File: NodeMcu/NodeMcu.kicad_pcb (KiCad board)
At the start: 2 copper layers, 8.2 x 5 mm, 38 parts, among them J1 Conn_01x15_Male, J2 Conn_01x15_Male, P1 USB_C_Plug_USB2.0, Q1 Q_Dual_NPN_NPN_E1B1C2E2B2C1, SW1 SW_Push, SW2 SW_Push, U1 ESP-12E, U2 SPX3819M5-L-3-3, U3 CH340C

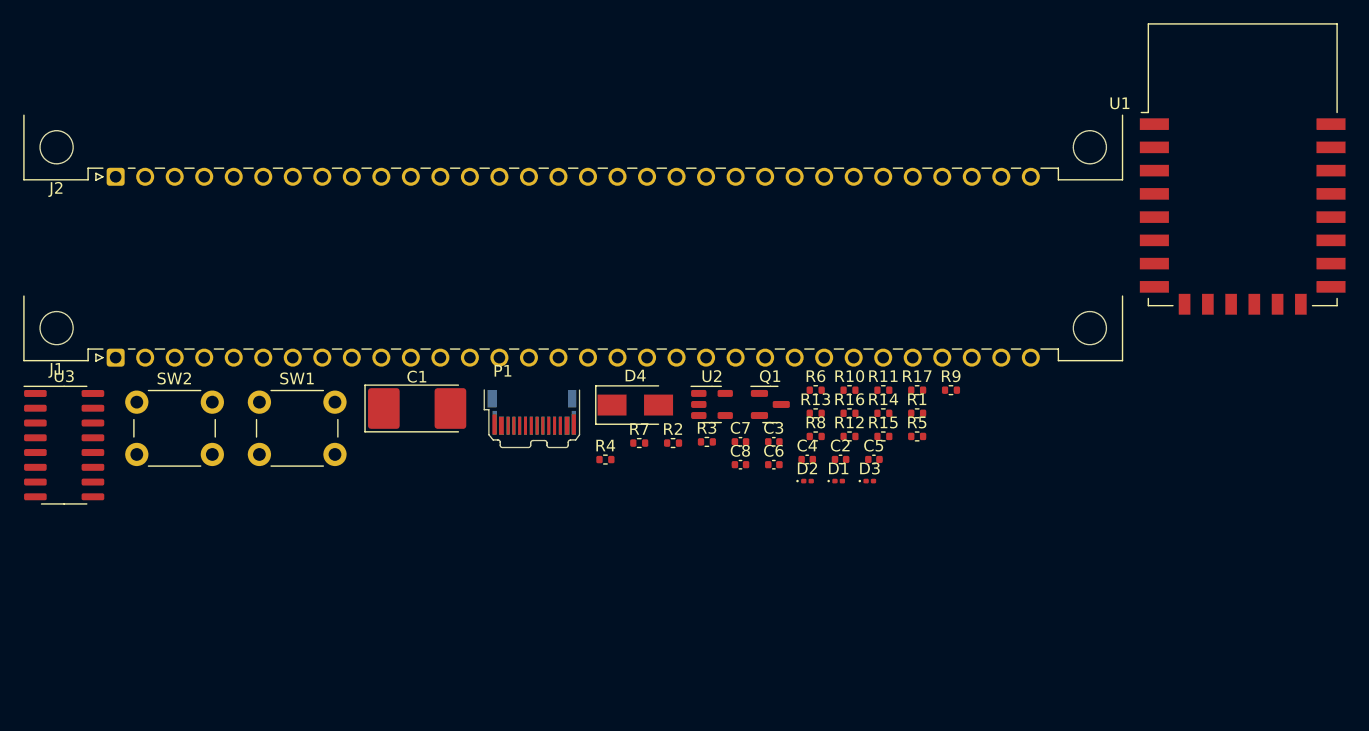
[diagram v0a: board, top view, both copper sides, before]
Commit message: nodemcu
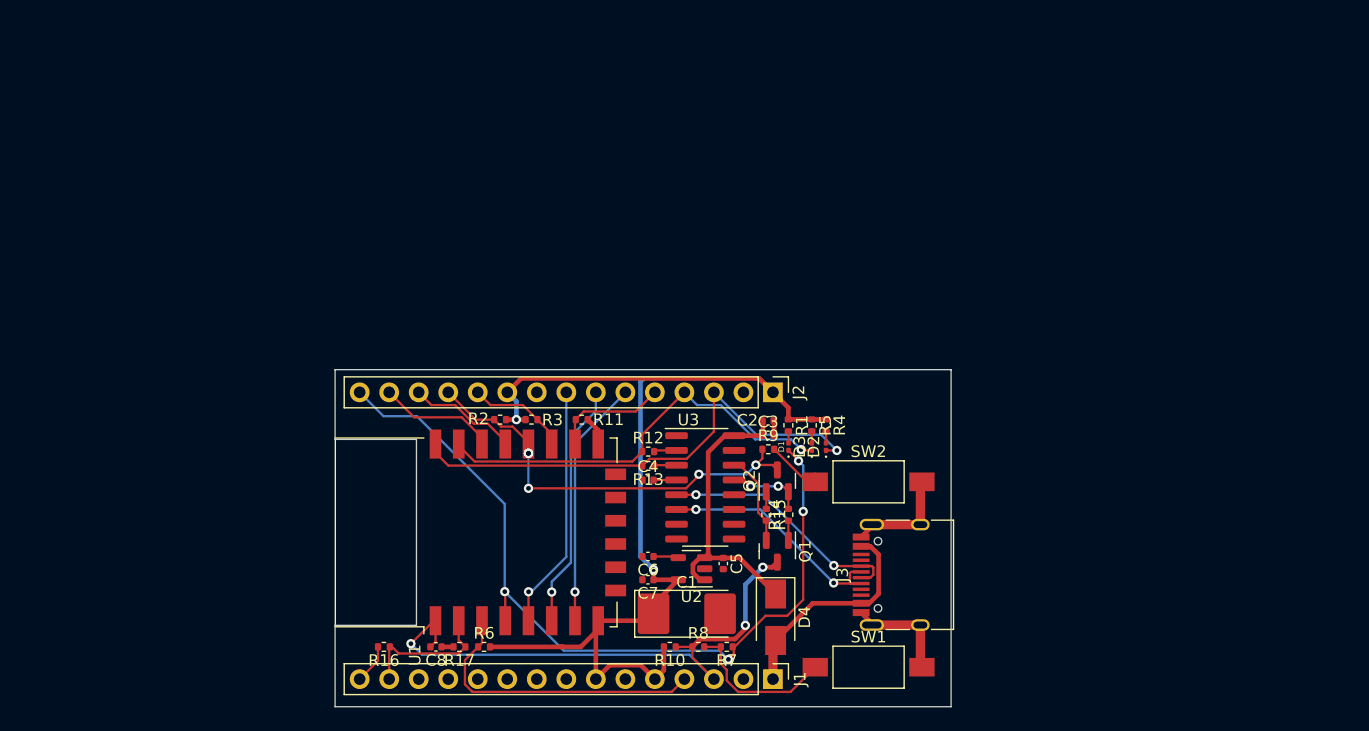
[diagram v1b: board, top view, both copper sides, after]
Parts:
- removed P1: USB_C_Plug_USB2.0, Connector_USB:USB_C_Plug_JAE_DX07P024AJ1
- added J3: USB_C_Receptacle_USB2.0, Connector_USB:USB_C_Receptacle_HRO_TYPE-C-31-M-12, F.Cu at (141.3, 67.7)
- added Q2: Q_NPN_BEC, Package_TO_SOT_SMD:SOT-23, F.Cu at (130.1, 59.6)
- J1, J2: footprint Connector_DIN:DIN41612_B_1x32_Male_Horizontal_THT -> Connector_PinHeader_2.54mm:PinHeader_1x15_P2.54mm_Vertical
- Q1: value Q_Dual_NPN_NPN_E1B1C2E2B2C1 -> Q_NPN_BEC
- SW1, SW2: footprint Button_Switch_THT:SW_PUSH_6mm -> Button_Switch_SMD:SW_SPST_FSMSM
- moved U1 73.1 mm to (104.1, 64.0), turned to 90 degrees
- moved SW2 63.3 mm to (137.9, 59.6)
- moved J1 63.0 mm to (129.7, 76.6), turned to -90 degrees
- moved J2 59.5 mm to (129.7, 52.0), turned to -90 degrees
- moved SW1 57.2 mm to (137.9, 75.6)
- moved U3 55.3 mm to (123.8, 60.1)
- moved R17 45.2 mm to (102.7, 73.8), turned to 180 degrees
- moved R16 44.8 mm to (96.2, 73.8), turned to 180 degrees
- moved R6 36.1 mm to (104.8, 73.8)
- moved C8 30.5 mm to (100.7, 73.8), turned to 180 degrees
- moved C1 29.2 mm to (122.3, 71.0)
- moved R10 27.0 mm to (120.8, 73.8), turned to 180 degrees
- moved R11 26.1 mm to (113.2, 54.3)
- moved D4 21.9 mm to (129.9, 71.3), turned to -90 degrees
- moved R8 20.7 mm to (123.2, 73.8)
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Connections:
- C1 pad 2: +3V3 -> GND
- C2 pad 2: +3V3 -> GND
- C3 pad 2: +3V3 -> GND
- C4 pad 1: +3V3 -> GND
- C5 pad 2: +3V3 -> GND
- C6 pad 2: +3V3 -> GND
- C7 pad 2: +3V3 -> GND
- C8 pad 1: +3V3 -> GND
- Q1 pad 3: /GPIO0 -> /nRST
- R11 pad 2: +3V3 -> GND
- R14 pad 1: Net-(Q1-Pad2) -> Net-(Q1-Pad1)
- R15 pad 2: Net-(Q1-Pad1) -> Net-(Q1-Pad2)
- R17 pad 2: +3V3 -> GND
- SW1 pad 2: +3V3 -> GND
- SW2 pad 2: +3V3 -> GND
- U1 pad 15: +3V3 -> GND
- U2 pad 2: +3V3 -> GND
- U3 pad 1: +3V3 -> GND
- U3 pad 14: Net-(Q1-Pad1) -> Net-(Q1-Pad2)
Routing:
- net +3V3: track 0.00 -> 100.1 mm, vias 0 -> 2
- net /GPIO16: track 0.00 -> 70.6 mm, vias 0 -> 4
- net /nRST: track 0.00 -> 50.2 mm, vias 0 -> 3
- net /TXD: track 0.00 -> 43.4 mm, vias 0 -> 1
- net /GPIO0: track 0.00 -> 36.7 mm, vias 0 -> 5
- net /RXD: track 0.00 -> 36.6 mm, vias 0 -> 1
- net +5VD: track 0.00 -> 26.4 mm
- net /EN: track 0.00 -> 25.7 mm
- net GND: track 0.00 -> 24.0 mm
- net /GPIO13: track 0.00 -> 21.5 mm, vias 0 -> 1
- net Net-(J3-PadA7): track 0.00 -> 21.4 mm, vias 0 -> 2
- net Net-(J3-PadA6): track 0.00 -> 21.3 mm, vias 0 -> 2
- net /GPIO12: track 0.00 -> 21.2 mm, vias 0 -> 1
- net /GPIO14: track 0.00 -> 21.1 mm, vias 0 -> 1
- net /VDDUSB: track 0.00 -> 19.1 mm
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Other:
- board size 8.2 x 5 mm -> 53 x 29 mm
